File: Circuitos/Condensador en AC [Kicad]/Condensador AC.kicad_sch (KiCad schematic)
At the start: 3 parts

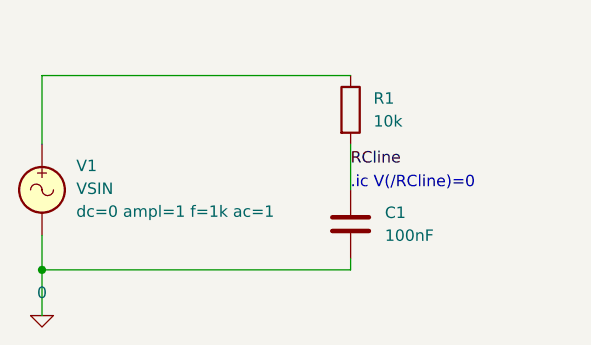
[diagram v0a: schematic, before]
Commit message: .
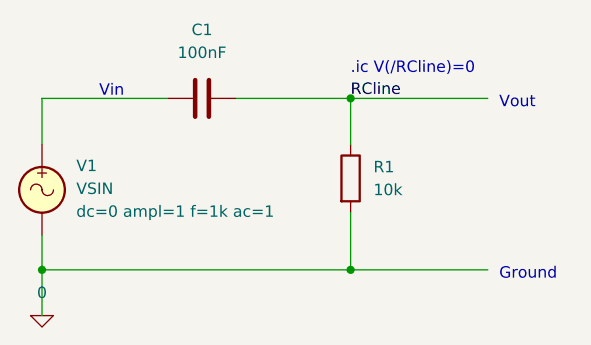
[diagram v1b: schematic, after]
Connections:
- net 0: now also R1.2; no longer C1.2
- net RCline: now also C1.2, R1.1; no longer C1.1, R1.2
- net at V1.1: now also C1.1; no longer R1.1
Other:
- note added: "Ground"
- note added: "Vin"
- note added: "Vout"
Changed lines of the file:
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@@
   (junction (at 120.65 100.33) (diameter 0) (color 0 0 0 0)
   )
-  (wire (pts (xy 154.94 99.06) (xy 154.94 100.33))
+  (junction (at 154.94 81.28) (diameter 0) (color 0 0 0 0)
+  )
+  (junction (at 154.94 100.33) (diameter 0) (color 0 0 0 0)
+  )
+  (wire (pts (xy 154.94 81.28) (xy 170.18 81.28))
+    (stroke (width 0) (type default))
+  )
+  (wire (pts (xy 154.94 100.33) (xy 170.18 100.33))
+    (stroke (width 0) (type default))
+  )
+  (wire (pts (xy 154.94 93.98) (xy 154.94 100.33))
     (stroke (width 0) (type default))
   )
@@
     (stroke (width 0) (type default))
   )
-  (wire (pts (xy 154.94 78.74) (xy 120.65 78.74))
+  (wire (pts (xy 120.65 81.28) (xy 134.62 81.28))
     (stroke (width 0) (type default))
   )
-  (wire (pts (xy 154.94 86.36) (xy 154.94 91.44))
+  (wire (pts (xy 142.24 81.28) (xy 154.94 81.28))
     (stroke (width 0) (type default))
   )
-  (wire (pts (xy 120.65 78.74) (xy 120.65 86.36))
+  (wire (pts (xy 154.94 81.28) (xy 154.94 86.36))
+    (stroke (width 0) (type default))
+  )
+  (wire (pts (xy 120.65 81.28) (xy 120.65 86.36))
     (stroke (width 0) (type default))
   )
@@
     (stroke (width 0) (type default))
   )
-  (text ".ic V(/RCline)=0" (at 154.94 91.44 0)
+  (text "Ground" (at 171.45 101.6 0)
     (effects (font (size 1.27 1.27)) (justify left bottom))
   )
-  (label "RCline" (at 154.94 88.9 0) (fields_autoplaced)
+  (text "Vout" (at 171.45 82.55 0)
+    (effects (font (size 1.27 1.27)) (justify left bottom))
+  )
+  (text "Vin" (at 127 81.28 0)
+    (effects (font (size 1.27 1.27)) (justify left bottom))
+  )
+  (text ".ic V(/RCline)=0" (at 154.94 78.74 0)
+    (effects (font (size 1.27 1.27)) (justify left bottom))
+  )
+  (label "RCline" (at 154.94 81.28 0) (fields_autoplaced)
     (effects (font (size 1.27 1.27)) (justify left bottom))
   )
@@
     )
   )
-  (symbol (lib_id "Device:C") (at 154.94 95.25 0) (unit 1)
+  (symbol (lib_id "Device:R") (at 154.94 90.17 0) (unit 1)
     (in_bom yes) (on_board yes) (dnp no) (fields_autoplaced)
-    (property "Reference" "C1" (at 158.75 93.98 0)
+    (property "Reference" "R1" (at 157.48 88.9 0)
       (effects (font (size 1.27 1.27)) (justify left))
     )
-    (property "Value" "100nF" (at 158.75 96.52 0)
+    (property "Value" "10k" (at 157.48 91.44 0)
       (effects (font (size 1.27 1.27)) (justify left))
     )
-    (property "Footprint" "" (at 155.9052 99.06 0)
+    (property "Footprint" "" (at 153.162 90.17 90)
       (effects (font (size 1.27 1.27)) hide)
     )
-    (property "Datasheet" "~" (at 154.94 95.25 0)
+    (property "Datasheet" "~" (at 154.94 90.17 0)
+      (effects (font (size 1.27 1.27)) hide)
+    )
+    (pin "2")
+    (pin "1")
+    (instances
+      (project "Condensador AC"
+        (path "/7e973ca0-a965-4a5b-b309-2418d7b47edb"
+          (reference "R1") (unit 1)
+        )
+      )
+      (project "Radio_1920"
+        (path "/bac7193f-7456-4028-8662-c026acd3ae4e"
+          (reference "R1") (unit 1)
+        )
+      )
+      (project "Carga condensador"
+        (path "/be4088d1-1f89-4bc2-a05e-f544ac528fd4"
+          (reference "R1") (unit 1)
+        )
+      )
+    )
+  )
+  (symbol (lib_id "Device:C") (at 138.43 81.28 90) (unit 1)
+    (in_bom yes) (on_board yes) (dnp no) (fields_autoplaced)
+    (property "Reference" "C1" (at 138.43 73.66 90)
+      (effects (font (size 1.27 1.27)))
+    )
+    (property "Value" "100nF" (at 138.43 76.2 90)
+      (effects (font (size 1.27 1.27)))
+    )
+    (property "Footprint" "" (at 142.24 80.3148 0)
+      (effects (font (size 1.27 1.27)) hide)
+    )
+    (property "Datasheet" "~" (at 138.43 81.28 0)
       (effects (font (size 1.27 1.27)) hide)
     )
@@
         )
       )
-    )
-  )
-  (symbol (lib_id "Device:R") (at 154.94 82.55 0) (unit 1)
-    (in_bom yes) (on_board yes) (dnp no) (fields_autoplaced)
-    (property "Reference" "R1" (at 157.48 81.28 0)
-      (effects (font (size 1.27 1.27)) (justify left))
-    )
-    (property "Value" "10k" (at 157.48 83.82 0)
-      (effects (font (size 1.27 1.27)) (justify left))
-    )
-    (property "Footprint" "" (at 153.162 82.55 90)
-      (effects (font (size 1.27 1.27)) hide)
-    )
-    (property "Datasheet" "~" (at 154.94 82.55 0)
-      (effects (font (size 1.27 1.27)) hide)
-    )
-    (pin "2")
-    (pin "1")
-    (instances
-      (project "Condensador AC"
-        (path "/7e973ca0-a965-4a5b-b309-2418d7b47edb"
-          (reference "R1") (unit 1)
-        )
-      )
-      (project "Radio_1920"
-        (path "/bac7193f-7456-4028-8662-c026acd3ae4e"
-          (reference "R1") (unit 1)
-        )
-      )
-      (project "Carga condensador"
-        (path "/be4088d1-1f89-4bc2-a05e-f544ac528fd4"
-          (reference "R1") (unit 1)
-        )
-      )
